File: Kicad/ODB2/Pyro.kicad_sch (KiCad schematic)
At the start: 33 parts, among them U11 TLV2372, U12 74LVC2G08GT_115, U13 TLV2372

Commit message: ajout footprints
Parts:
- Pyros_LED1, Pyros_LED2, Pyros_LED3: footprint (none) -> LED_SMD:LED_0805_2012Metric
- Pyros_R1, Pyros_R10, Pyros_R11, Pyros_R12, Pyros_R13, Pyros_R14, Pyros_R15, Pyros_R16, Pyros_R17, Pyros_R18, Pyros_R19, Pyros_R2, Pyros_R3, Pyros_R4, Pyros_R5, Pyros_R6, Pyros_R7, Pyros_R8, Pyros_R9: footprint (none) -> Resistor_SMD:R_0805_2012Metric
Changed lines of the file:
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@@
 			)
 		)
-		(property "Footprint" ""
+		(property "Footprint" "Resistor_SMD:R_0805_2012Metric"
 			(at 166.37 36.322 90)
 			(effects
@@
 			)
 		)
-		(property "Footprint" ""
+		(property "Footprint" "LED_SMD:LED_0805_2012Metric"
 			(at 95.25 176.53 0)
 			(effects
@@
 			)
 		)
-		(property "Footprint" ""
+		(property "Footprint" "Resistor_SMD:R_0805_2012Metric"
 			(at 151.13 97.282 90)
 			(effects
@@
 			)
 		)
-		(property "Footprint" ""
+		(property "Footprint" "Resistor_SMD:R_0805_2012Metric"
 			(at 41.91 96.012 90)
 			(effects
@@
 			)
 		)
-		(property "Footprint" ""
+		(property "Footprint" "Resistor_SMD:R_0805_2012Metric"
 			(at 56.388 72.39 90)
 			(effects
@@
 			)
 		)
-		(property "Footprint" ""
+		(property "Footprint" "Resistor_SMD:R_0805_2012Metric"
 			(at 71.882 82.55 90)
 			(effects
@@
 			)
 		)
-		(property "Footprint" ""
+		(property "Footprint" "Resistor_SMD:R_0805_2012Metric"
 			(at 173.228 43.18 90)
 			(effects
@@
 			)
 		)
-		(property "Footprint" ""
+		(property "Footprint" "Resistor_SMD:R_0805_2012Metric"
 			(at 50.038 104.14 90)
 			(effects
@@
 			)
 		)
-		(property "Footprint" ""
+		(property "Footprint" "Resistor_SMD:R_0805_2012Metric"
 			(at 181.102 83.82 90)
 			(effects
@@
 			)
 		)
-		(property "Footprint" ""
+		(property "Footprint" "Resistor_SMD:R_0805_2012Metric"
 			(at 168.148 109.22 90)
 			(effects
@@
 			)
 		)
-		(property "Footprint" ""
+		(property "Footprint" "Resistor_SMD:R_0805_2012Metric"
 			(at 58.928 107.95 90)
 			(effects
@@
 			)
 		)
-		(property "Footprint" ""
+		(property "Footprint" "Resistor_SMD:R_0805_2012Metric"
 			(at 165.608 73.66 90)
 			(effects
@@
 			)
 		)
-		(property "Footprint" ""
+		(property "Footprint" "Resistor_SMD:R_0805_2012Metric"
 			(at 57.15 35.052 90)
 			(effects
@@
 			)
 		)
-		(property "Footprint" ""
+		(property "Footprint" "Resistor_SMD:R_0805_2012Metric"
 			(at 41.91 174.752 90)
 			(effects
@@
 			)
 		)
-		(property "Footprint" ""
+		(property "Footprint" "LED_SMD:LED_0805_2012Metric"
 			(at 52.07 176.53 0)
 			(effects
@@
 			)
 		)
-		(property "Footprint" ""
+		(property "Footprint" "Resistor_SMD:R_0805_2012Metric"
 			(at 78.74 57.658 90)
 			(effects
@@
 			)
 		)
-		(property "Footprint" ""
+		(property "Footprint" "Resistor_SMD:R_0805_2012Metric"
 			(at 64.008 41.91 90)
 			(effects
@@
 			)
 		)
-		(property "Footprint" ""
+		(property "Footprint" "Resistor_SMD:R_0805_2012Metric"
 			(at 187.96 58.928 90)
 			(effects
@@
 			)
 		)
-		(property "Footprint" ""
+		(property "Footprint" "Resistor_SMD:R_0805_2012Metric"
 			(at 129.54 174.752 90)
 			(effects
@@
 			)
 		)
-		(property "Footprint" ""
+		(property "Footprint" "Resistor_SMD:R_0805_2012Metric"
 			(at 85.09 174.752 90)
 			(effects
@@
 			)
 		)
-		(property "Footprint" ""
+		(property "Footprint" "Resistor_SMD:R_0805_2012Metric"
 			(at 159.258 105.41 90)
 			(effects
@@
 			)
 		)
-		(property "Footprint" ""
+		(property "Footprint" "LED_SMD:LED_0805_2012Metric"
 			(at 139.7 176.53 0)
 			(effects

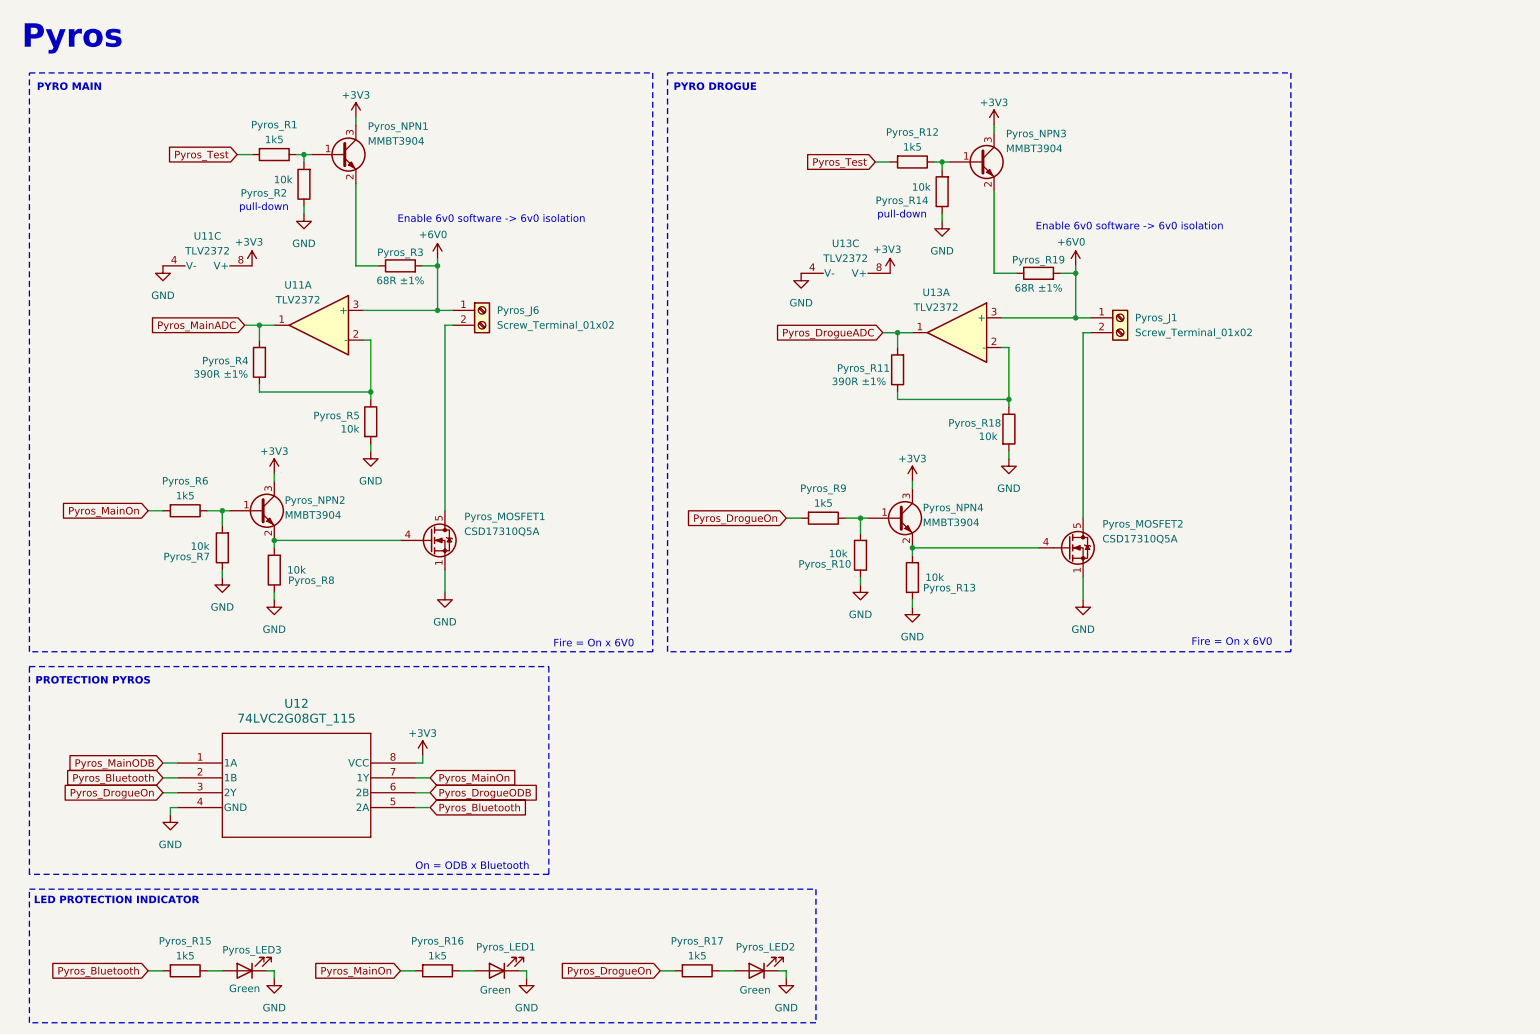
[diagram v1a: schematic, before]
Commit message: revision logic
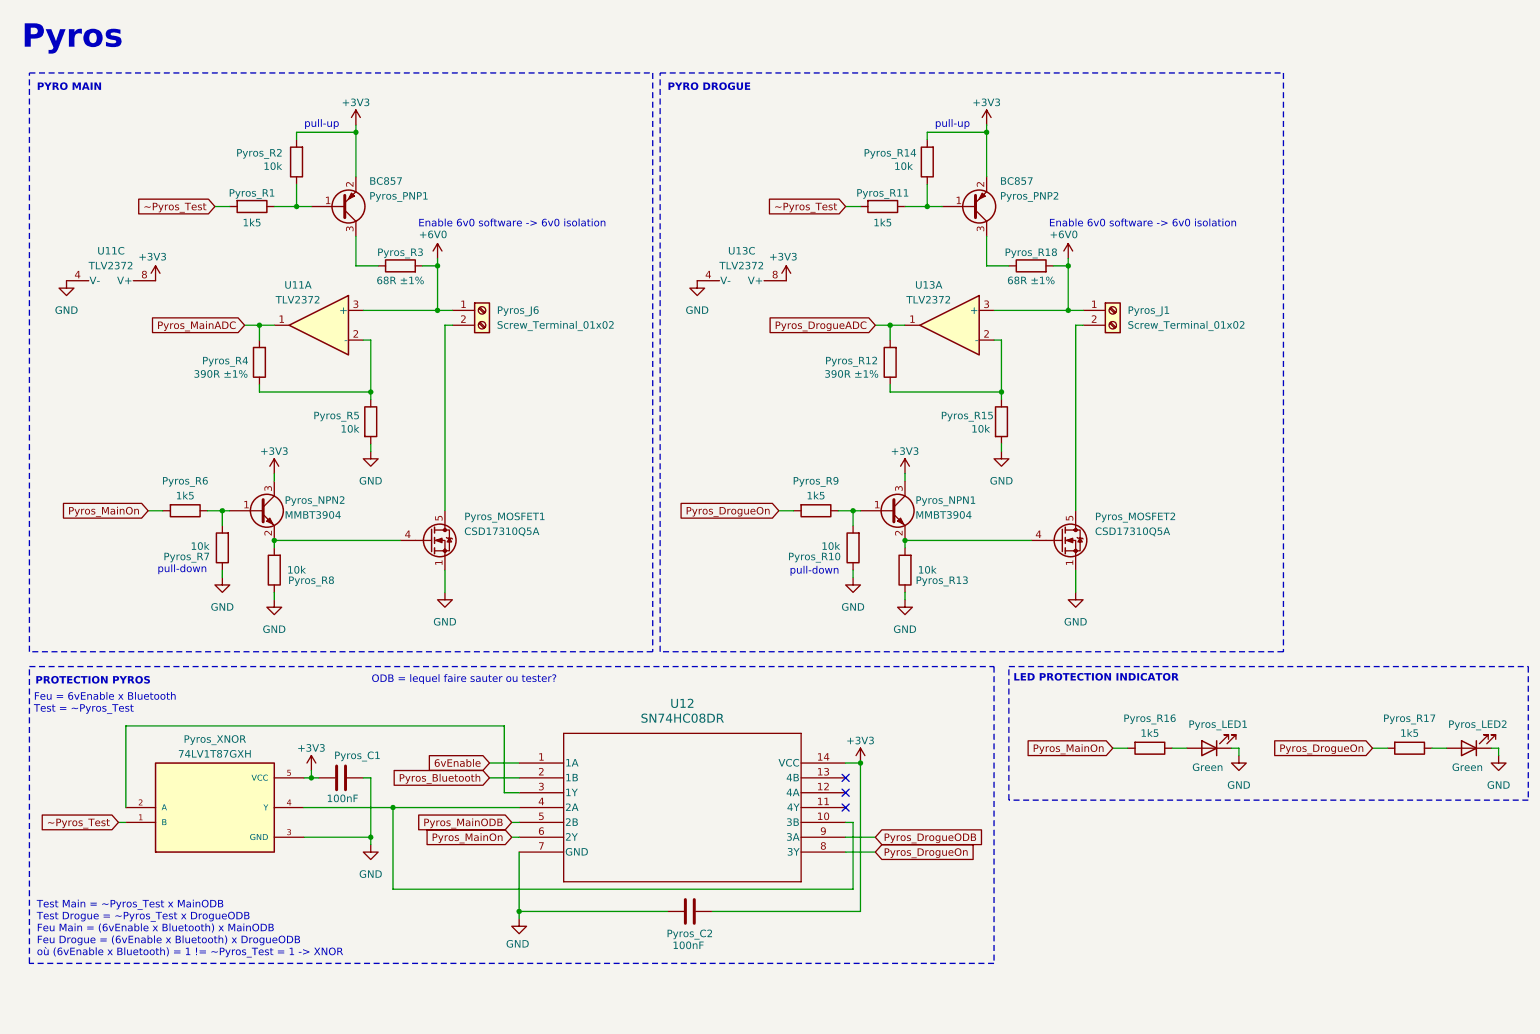
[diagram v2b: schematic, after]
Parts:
- removed Pyros_LED3: Green, LED_SMD:LED_0805_2012Metric, symbol Device:LED
- removed Pyros_NPN3, Pyros_NPN4: MMBT3904, Package_TO_SOT_SMD:SOT-23, symbol Transistor_BJT:MMBT3904
- removed Pyros_R19: 68R ±1%, Resistor_SMD:R_0805_2012Metric, symbol Device:R
- removed U12: 74LVC2G08GT_115, Library:XSON8_SOT833-1_NEX, symbol ODB_Lib:74LVC2G08GT_115
- added Pyros_C1, Pyros_C2: 100nF, symbol Device:C
- added Pyros_PNP1, Pyros_PNP2: BC857, Package_TO_SOT_SMD:SOT-23, symbol Transistor_BJT:BC857
- added Pyros_XNOR: 74LV1T87GXH, 74LV1T87GXH:IC_74LV1T87GXH, symbol ODB_Lib:74LV1T87GXH
- added U12: SN74HC08DR, D14, symbol ODB_Lib:SN74HC08DR
- Pyros_R11: value 390R ±1% -> 1k5
- Pyros_R12: value 1k5 -> 390R ±1%
- Pyros_R15: value 1k5 -> 10k
- Pyros_R18: value 10k -> 68R ±1%
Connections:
- net +3V3: now also Pyros_R14.2, Pyros_R2.2, Pyros_C1.2, Pyros_C2.1, Pyros_PNP1.2 (E), Pyros_PNP2.2 (E), Pyros_XNOR.5 (VCC), U12.14 (VCC)
- net +6V0: now also Pyros_R18.2
- net GND: now also Pyros_R15.2, Pyros_C1.1, Pyros_C2.2, Pyros_XNOR.3 (GND), U12.7 (GND); no longer Pyros_R14.1, Pyros_R18.2, Pyros_R2.1
- net Pyros_Bluetooth: now also U12.2 (1B); no longer Pyros_R15.2
- net Pyros_DrogueADC: now also Pyros_R12.2; no longer Pyros_R11.2
- net Pyros_DrogueODB: now also U12.9 (3A)
- net Pyros_DrogueOn: now also U12.8 (3Y)
- net Pyros_MainODB: now also U12.5 (2B)
- net Pyros_MainOn: now also U12.6 (2Y)
- net at Pyros_R12.1: now also Pyros_R15.1, U13.2 (-); no longer Pyros_R14.2
- net at Pyros_R10.2, Pyros_R9.1: now also Pyros_NPN1.1 (B)
- net at Pyros_MOSFET2.4 (G), Pyros_R13.2: now also Pyros_NPN1.2 (E)
- net at Pyros_R3.1: now also Pyros_PNP1.3 (C); no longer Pyros_NPN1.2 (E)
- net Pyros_Test renamed ~Pyros_Test
- net ~Pyros_Test: now also Pyros_R11.2, Pyros_XNOR.1 (B); no longer Pyros_R12.2
- new net: Pyros_PNP1.1 (B), Pyros_R1.1, Pyros_R2.1
- new net: Pyros_PNP2.3 (C), Pyros_R18.1
- new net: Pyros_PNP2.1 (B), Pyros_R11.1, Pyros_R14.1
- new net: Pyros_XNOR.2 (A), U12.3 (1Y)
- new net: Pyros_XNOR.4 (Y), U12.10 (3B), U12.4 (2A)
- new net 6vEnable: U12.1 (1A)
- no-connect marks 0 -> 3
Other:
- note added: "Feu = 6vEnable x Bluetooth Test = ~Pyros_Test"
- note added: "ODB = lequel faire sauter ou tester?"
- note added: "Test Main = ~Pyros_Test x MainODB Test Drogue = ~Pyros_Test x DrogueODB Feu Main = (6vEnable x Bluetooth) x MainODB Feu Drogue = (6vEnable x Bluetooth) x DrogueODB où (6vEnable x Bluetooth) = 1 != ~Pyros_Test = 1 -> XNOR"
- note added: "pull-up"
- note removed: "Fire = On x 6V0"
- note removed: "On = ODB x Bluetooth"
- moved on the sheet: Pyros_LED1, Pyros_LED2, Pyros_R1, Pyros_R16, Pyros_R17, U11C
